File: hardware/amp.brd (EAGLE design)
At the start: 100 x 100 mm, 37 parts, among them X1 2508-5

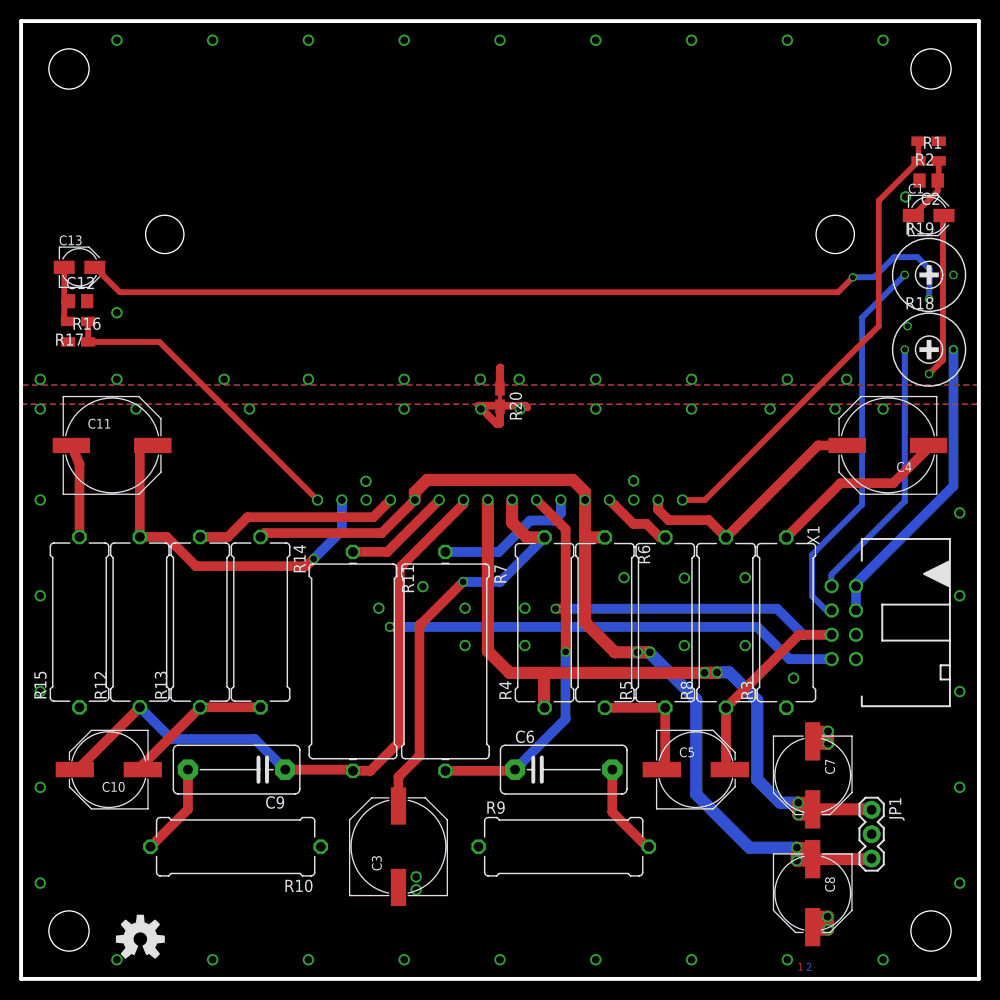
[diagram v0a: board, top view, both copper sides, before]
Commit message: board rev 1.1
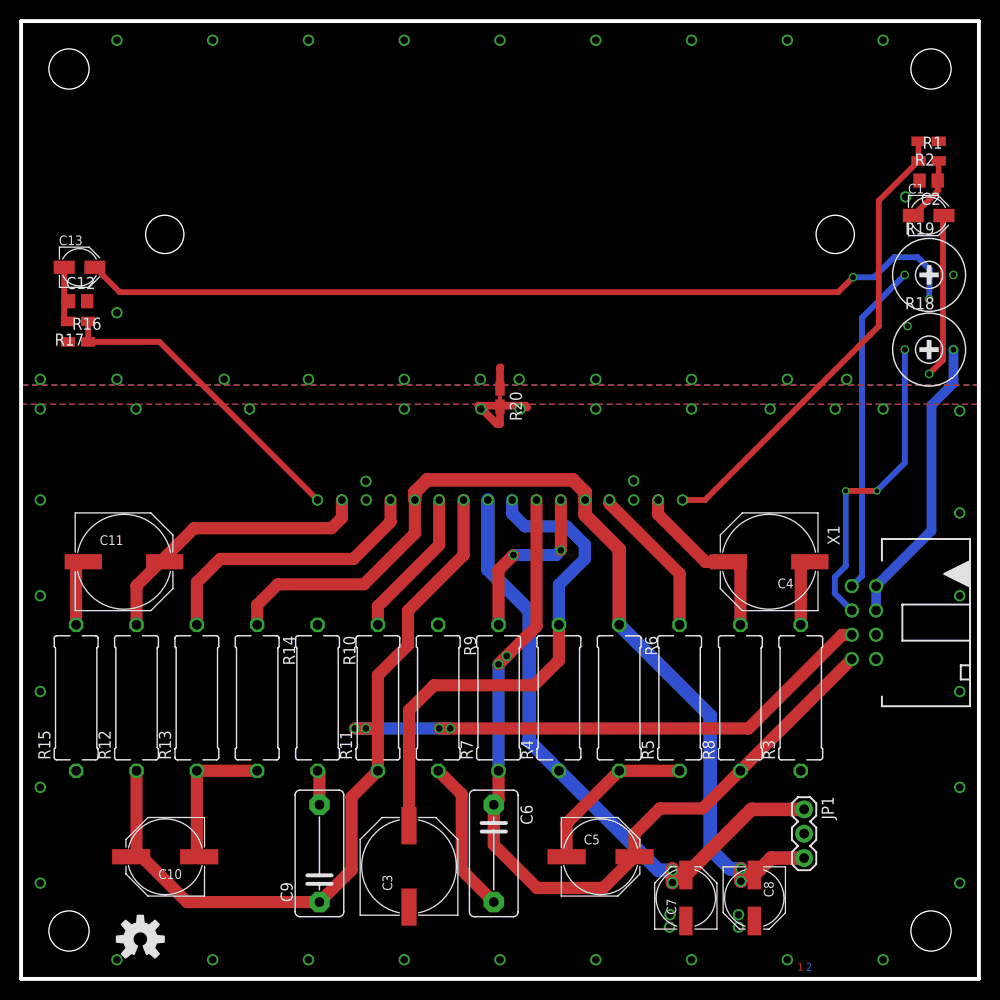
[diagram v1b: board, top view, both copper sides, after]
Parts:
- C7, C8: device rcl:PANASONIC_F -> rcl:PANASONIC_D
- R10, R12, R13, R14, R15, R3, R4, R5, R6, R8, R9: device rcl:0617/17 -> rcl:P0613/15
- R11, R7: device rcl:0922/22 -> rcl:P0613/15
- moved R9 20.3 mm to (43.5, 29.4), turned to 270 degrees
- moved C7 18.4 mm to (69.4, 8.45), turned to 90 degrees
- moved R10 17.7 mm to (30.9, 29.4), turned to 270 degrees
- moved C4 17.4 mm to (78.1, 43.5)
- moved C5 13.5 mm to (60.5, 12.8)
- moved C9 12.3 mm to (31.1, 13.1), turned to 90 degrees
- moved C11 12.2 mm to (10.8, 43.5)
- moved C6 11.4 mm to (49.4, 13.1), turned to 270 degrees
- moved C10 10.8 mm to (15.1, 12.8)
- moved R3 7.99 mm to (81.4, 29.4)
- moved R4 7.99 mm to (56.1, 29.4)
- moved R5 7.99 mm to (68.8, 29.4)
- moved R6 7.99 mm to (62.5, 29.4)
- moved R8 7.99 mm to (75.1, 29.4)
- moved R12 7.91 mm to (12.1, 29.4)
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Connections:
- net IN_L: now also X1.3; no longer X1.1
- net IN_R: now also X1.1; no longer X1.3
- net N$12: now also R11.2; no longer R11.1
- net N$5: now also R7.2; no longer R7.1
- net OUT_L: now also R7.1, X1.7; no longer R7.2, X1.5
- net OUT_R: now also R11.1, X1.5; no longer R11.2, X1.7
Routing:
- net OUT_R: track 117.2 -> 138.2 mm, vias 1 -> 4
- net GND: track 25.2 -> 10.0 mm, vias 50 -> 37
- net N$1: track 19.0 -> 7.18 mm
- net N$6: track 43.4 -> 53.4 mm, vias 1 -> 0
- net +24V: track 76.9 -> 67.3 mm, vias 4 -> 2
- net N$7: track 7.44 -> 16.1 mm
- net N$19: track 21.5 -> 29.5 mm
- net N$2: track 25.9 -> 18.3 mm
- net N$17: track 37.8 -> 30.7 mm, vias 1 -> 0
- net N$4: track 9.75 -> 16.1 mm
- net -24V: track 108.2 -> 102.1 mm, vias 4 -> 2
- net N$20: track 9.67 -> 3.63 mm
- net IN_R: track 40.2 -> 34.8 mm
- net IN_L: track 27.9 -> 32.9 mm, vias 0 -> 2
- net N$3: track 12.9 -> 17.6 mm
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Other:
- board text added: "2x25W amplifier circuit rev 1.1 github.com/rodan/ampy author: petre rodan date: apr 2014"
- board text added: "IO IN_R GND IN_L GND OUT_R GND OUT_L GND"
- board text removed: "2x15W amplifier circuit rev 1.0 github.com/rodan/ampy author: petre rodan date: apr 2014"
- board text removed: "IO IN_L GND IN_R GND OUT_L GND OUT_R GND"
